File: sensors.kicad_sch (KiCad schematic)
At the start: 18 parts, among them J1 Amphenol_901-144, J2 Amphenol_901-144, Q8 IRLML2803, Q9 NDS8434, U2 BMM150, U3 BMI270, U4 S1216V8, U5 EP2W+

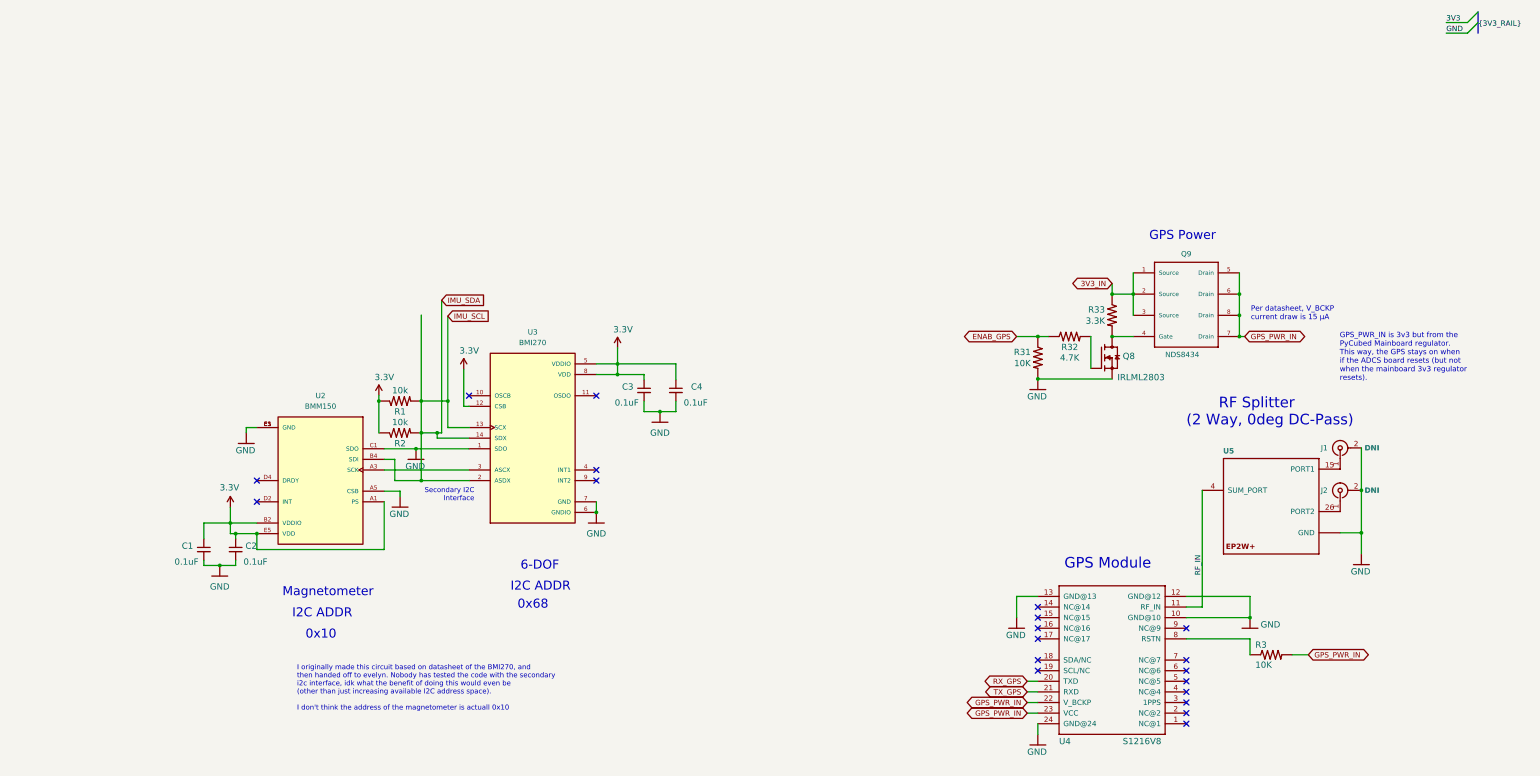
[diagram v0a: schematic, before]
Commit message: organize
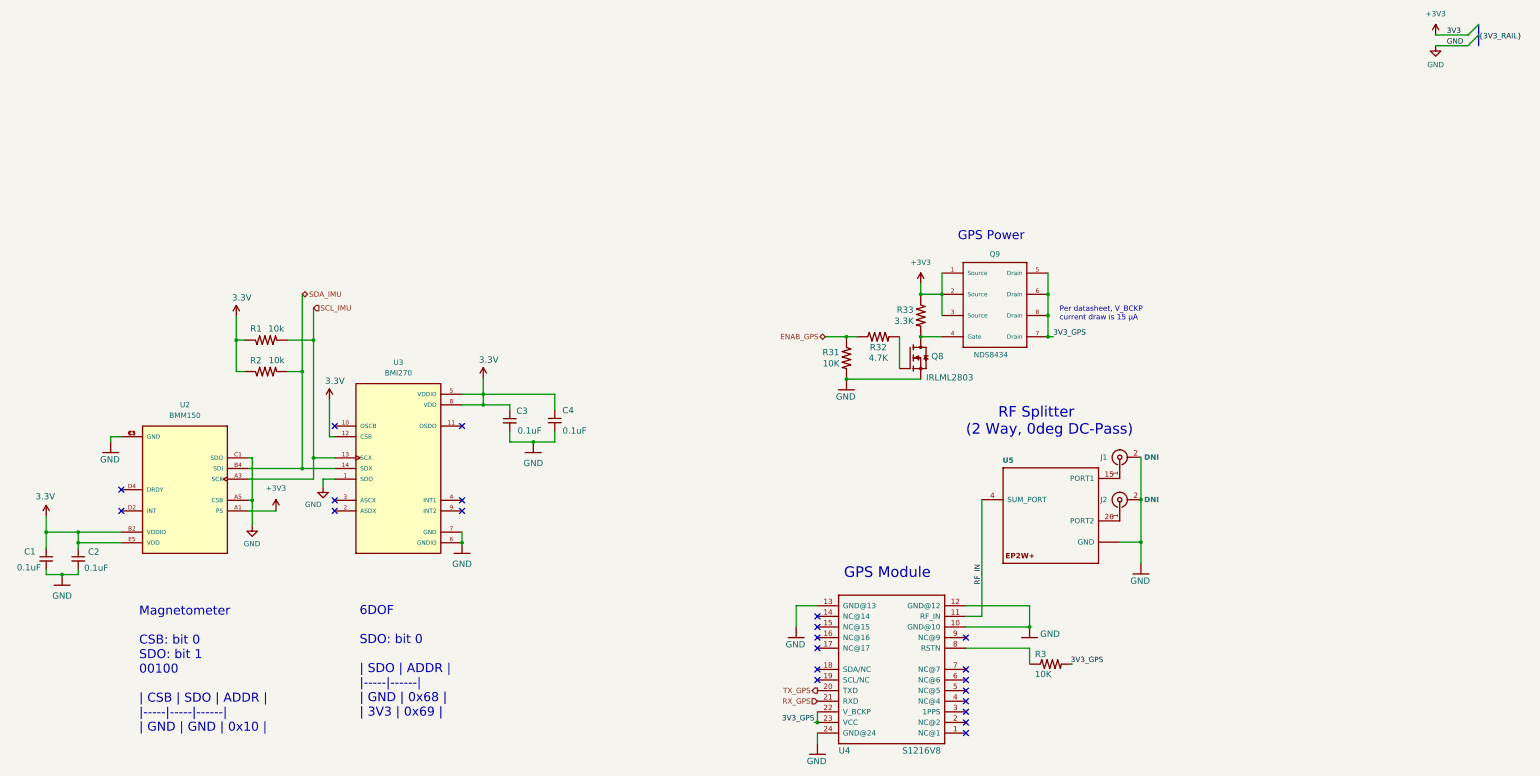
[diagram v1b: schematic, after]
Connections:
- net 3.3V: no longer U2.A1 (PS)
- net RX_GPS: now also U4.21 (RXD); no longer U4.20 (TXD)
- net TX_GPS: now also U4.20 (TXD); no longer U4.21 (RXD)
- net at U3.3 (ASCX): no longer U2.A3 (SCK)
- net 3V3_IN renamed +3V3
- net +3V3: now also U2.A1 (PS)
- net GPS_PWR_IN renamed 3V3_GPS
- net IMU_SCL renamed SDA_IMU
- net SDA_IMU: no longer R1.2, U3.13 (SCX), U3.2 (ASDX)
- new net SCL_IMU: R1.2, U2.A3 (SCK), U3.13 (SCX)
- no-connect marks 20 -> 22
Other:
- note added: "6DOF SDO: bit 0 | SDO | ADDR | |-----|------| | GND | 0x68 | | 3V3 | 0x69 |"
- note added: "Magnetometer CSB: bit 0 SDO: bit 1 00100 | CSB | SDO | ADDR | |-----|-----|------| | GND | GND | 0x10 |"
- note removed: "0x10"
- note removed: "0x68"
- note removed: "6-DOF"
- note removed: "GPS_PWR_IN is 3v3 but from the PyCubed Mainboard regulator. This way, the GPS stays on when if the ADCS board resets (but not when the mainboard 3v3 regulator resets)."
- note removed: "I originally made this circuit based on datasheet of the BMI270, and then handed off to evelyn. Nobody has tested the code with the secondary i2c interface, idk what the benefit of doing this would even be (other than just increasing available I2C address space). I don't think the address of the magnetometer is actuall 0x10"
- note removed: "I2C ADDR"
- note removed: "Magnetometer"
- note removed: "Secondary I2C Interface"
- moved on the sheet: C1, C2, C3, C4, J1, J2, Q8, Q9, R1, R2, R3, R31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

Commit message: ready for review
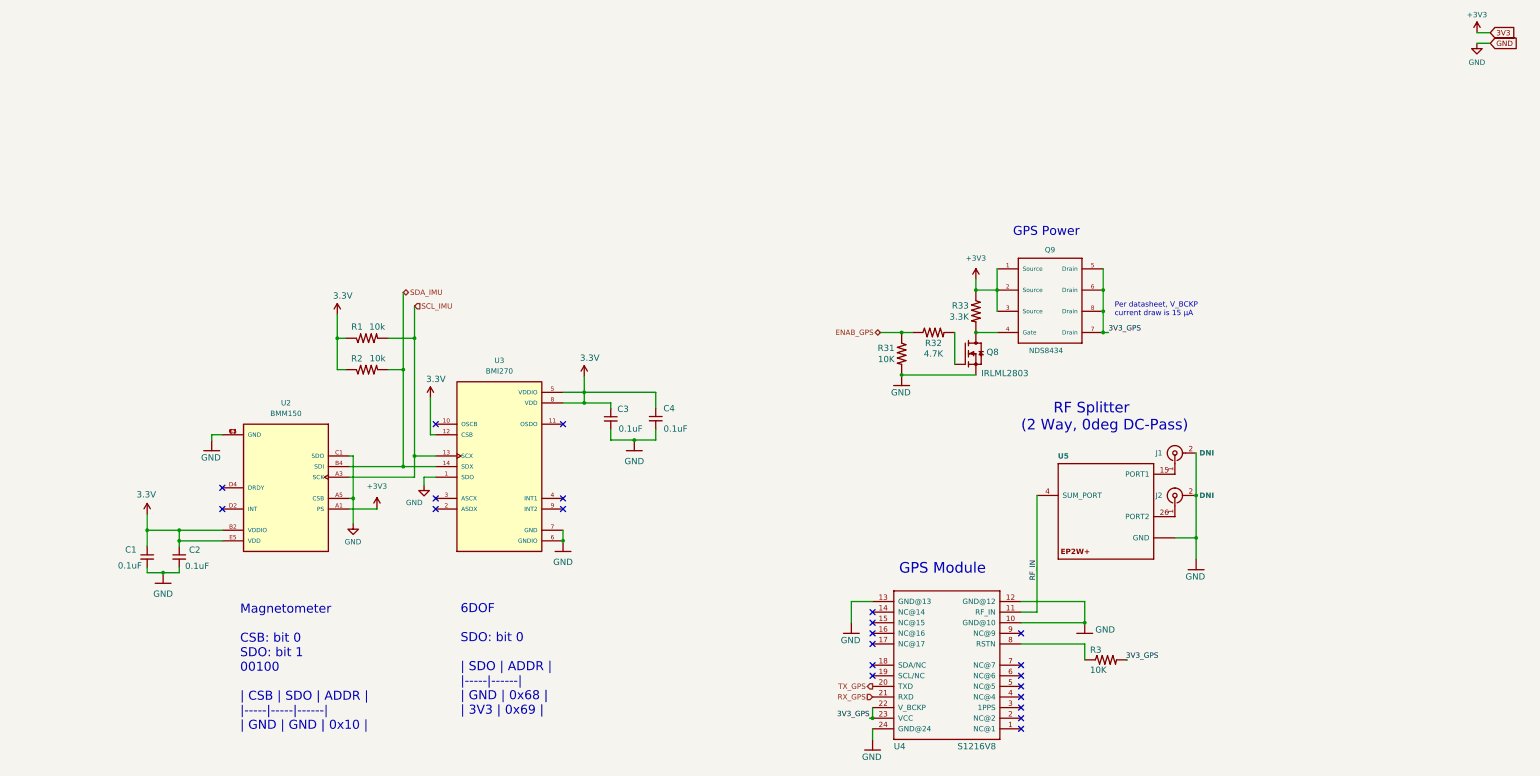
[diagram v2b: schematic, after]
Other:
- moved on the sheet: C1, C2, C3, C4, J1, J2, Q8, Q9, R1, R2, R3, R31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
